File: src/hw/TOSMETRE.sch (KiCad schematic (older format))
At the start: 26 parts, among them J1 Alim, J2 Conn_Coaxial, J3 PRG PIC, J4 LCD 4x20, J5 Conn_Coaxial, U1 18F1320, U2 L7805

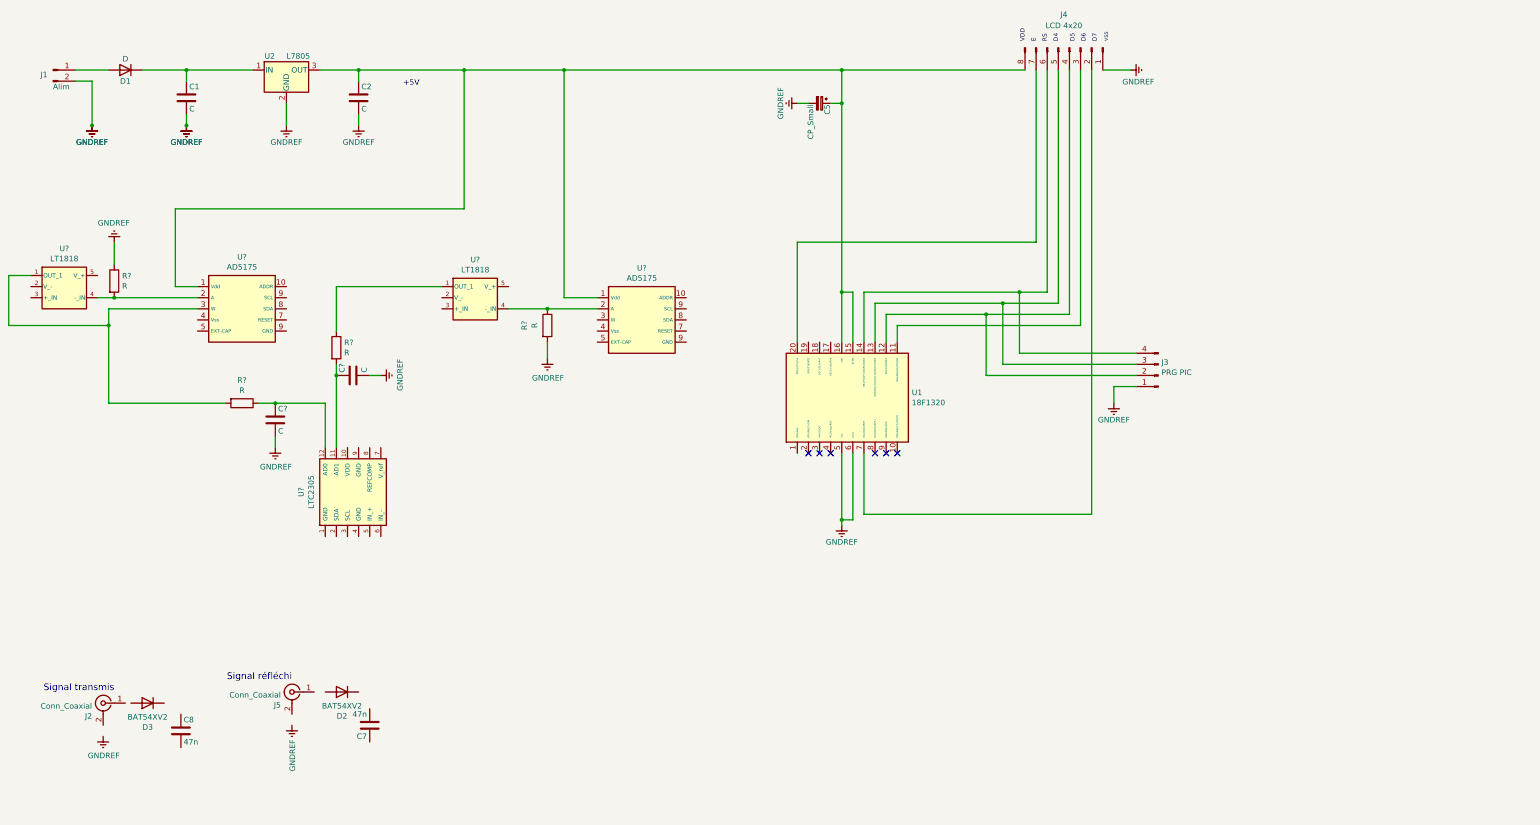
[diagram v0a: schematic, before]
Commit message: Raccordement AD LTC et LT suite
Raccordement AD LTC  et LT #196  mais maintenant je calle grave je me perd
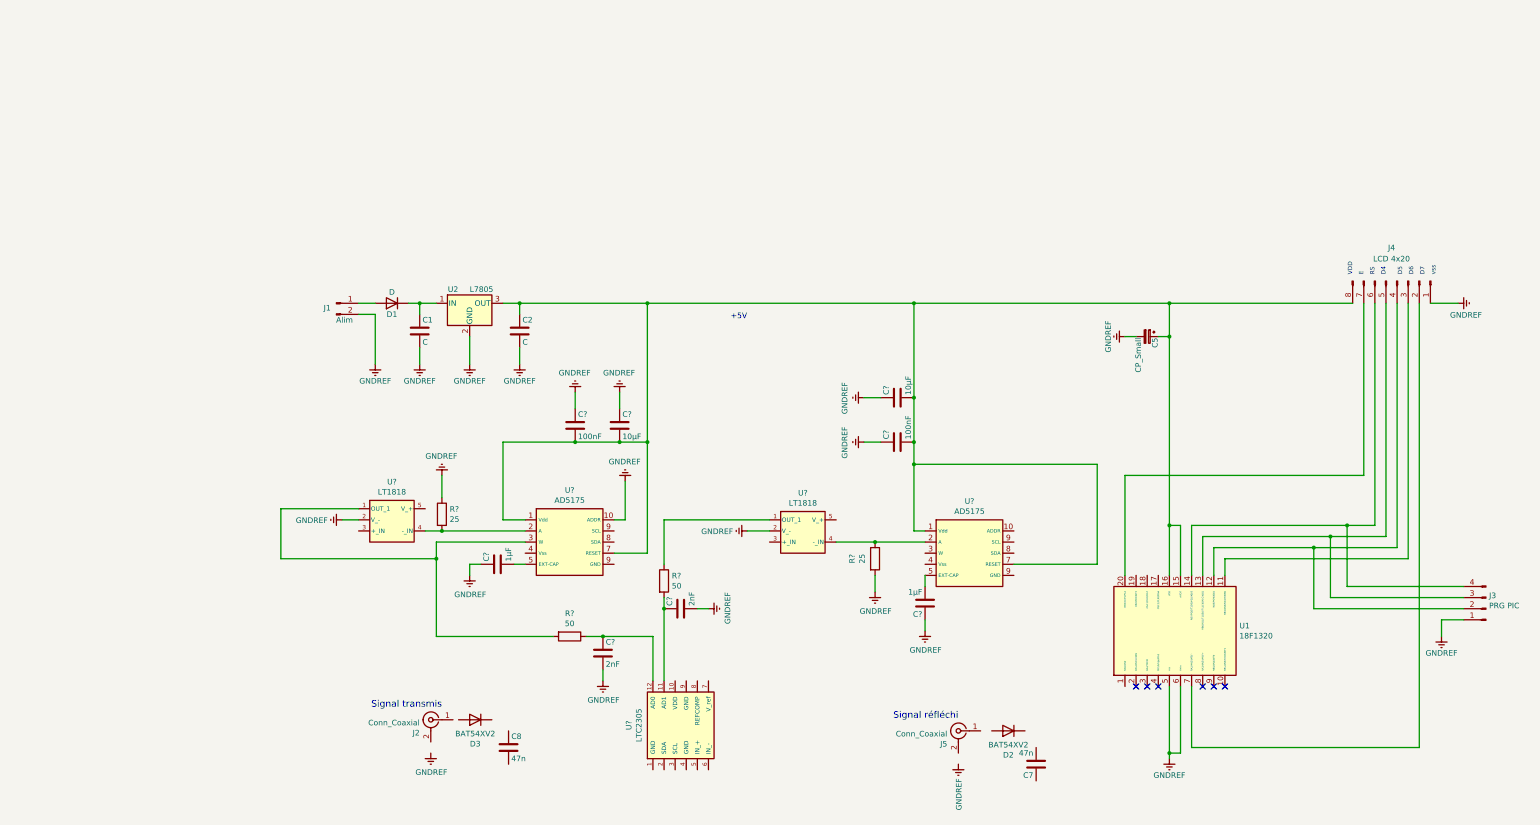
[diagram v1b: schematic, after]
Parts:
- added C? (x2): 1µF, Capacitor_SMD:C_1206_3216Metric, symbol Device:C
- added C? (x2): 10µF, Capacitor_SMD:C_1206_3216Metric, symbol Device:C
- added C? (x2): 100nF, Capacitor_SMD:C_1206_3216Metric, symbol Device:C
- C? (x2): value C -> 2nF
- R? (x2): value R -> 50
- R? (x2): value R -> 25
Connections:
- net GNDREF: now also U?.10 (ADDR), U?.2 (V_-), U?.2 (V_-), C?.1, C?.1, C?.1, C?.1, C?.1, C?.1
- net at C2.1, C5.1, J4.8 (Pin_8)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: now also U?.7 (RESET), U?.7 (RESET), C?.2, C?.2, C?.2, C?.2
- net at U?.5 (EXT-CAP): now also C?.2 (x2)
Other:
- moved on the sheet: C1, C2, C5, C7, C8, C?, D1, D2, D3, J1, J2, J3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
